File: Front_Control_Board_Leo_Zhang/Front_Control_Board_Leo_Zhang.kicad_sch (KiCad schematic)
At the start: 95 parts, among them J1 22035035, J10 430450200, J11 430450200, J12 430450200, J2 Molex Micro-Fit 4 Pin, J3 430450200, J4 430450200, J5 430450200, J6 430450200, J7 22035035, J8 22035035, J9 22035035, Q1 PSMN5R2-60YL, Q2 PSMN5R2-60YL, Q3 PSMN5R2-60YL, Q4 PSMN5R2-60YL, Q5 PSMN5R2-60YL, Q6 PSMN5R2-60YL, U2 ADS1118IDGS, U3 MCP2562-E-P, U5 UA78M05QDCYRG4Q1

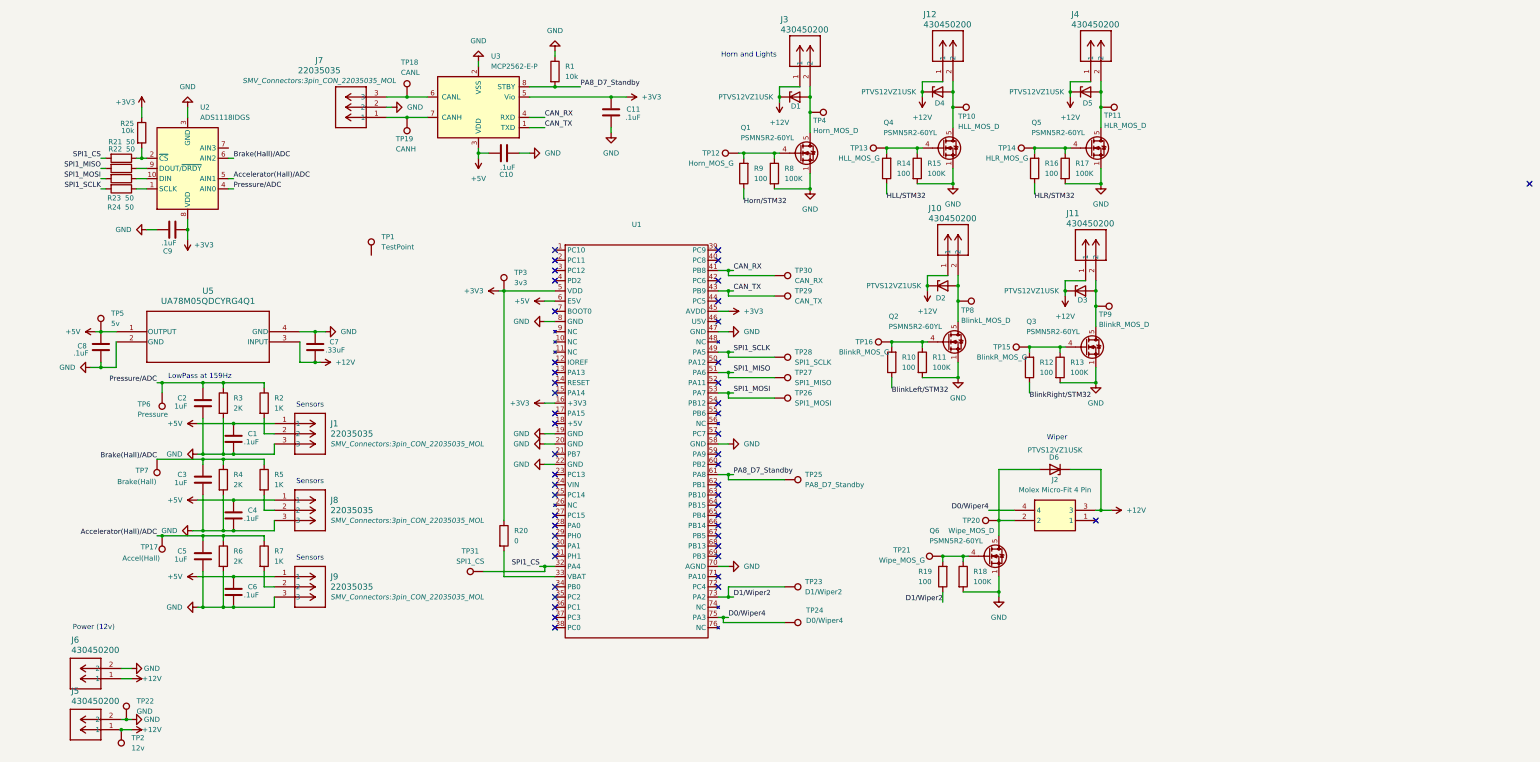
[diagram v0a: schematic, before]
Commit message: implemented initial feedback
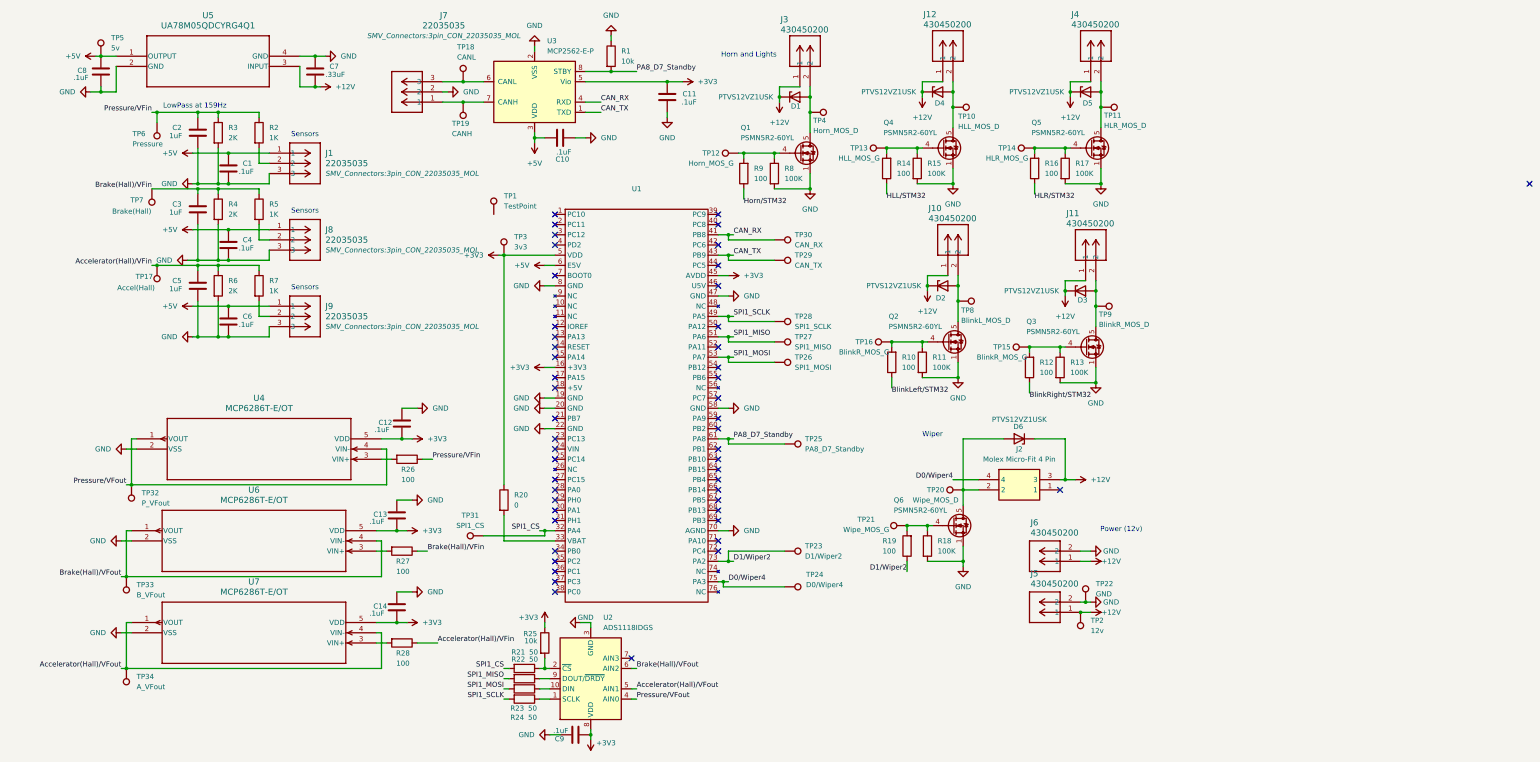
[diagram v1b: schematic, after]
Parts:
- added C12, C13, C14: .1uF, symbol Device:C
- added R26, R27, R28: 100, symbol Device:R
- added TP32: P_VFout, TestPoint:TestPoint_Pad_D1.0mm, symbol Connector:TestPoint
- added TP33: B_VFout, TestPoint:TestPoint_Pad_D1.0mm, symbol Connector:TestPoint
- added TP34: A_VFout, TestPoint:TestPoint_Pad_D1.0mm, symbol Connector:TestPoint
- added U4, U6, U7: MCP6286T-E/OT, SMV_ICs:SOT-23-5_MC_MCH, symbol SMV_Custom:MCP6286T-E_OT
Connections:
- net +3V3: now also C12.2, C13.2, C14.2, U4.5 (VDD), U6.5 (VDD), U7.5 (VDD)
- net GND: now also C12.1, C13.1, C14.1, U4.2 (VSS), U6.2 (VSS), U7.2 (VSS)
- net Accelerator(Hall)/ADC renamed Accelerator(Hall)/VFin
- net Accelerator(Hall)/VFin: now also R28.1; no longer U2.5 (AIN1)
- net Brake(Hall)/ADC renamed Brake(Hall)/VFin
- net Brake(Hall)/VFin: now also R27.1; no longer U2.6 (AIN2)
- net Pressure/ADC renamed Pressure/VFin
- net Pressure/VFin: now also R26.1; no longer U2.4 (AIN0)
- new net: R28.2, U7.3 (VIN+)
- new net: R26.2, U4.3 (VIN+)
- new net: R27.2, U6.3 (VIN+)
- new net Accelerator(Hall)/VFout: TP34.1, U2.5 (AIN1), U7.1 (VOUT), U7.4 (VIN-)
- new net Brake(Hall)/VFout: TP33.1, U2.6 (AIN2), U6.1 (VOUT), U6.4 (VIN-)
- new net Pressure/VFout: TP32.1, U2.4 (AIN0), U4.1 (VOUT), U4.4 (VIN-)
- no-connect marks 49 -> 50
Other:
- moved on the sheet: C1, C10, C11, C2, C3, C4, C5, C6, C7, C8, C9, D6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
